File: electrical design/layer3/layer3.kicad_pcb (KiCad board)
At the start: 2 copper layers, 150 x 140 mm, 58 parts, among them J1 XT60PW-M, J10 SH1.0 Female, J11 SH1.0 Female, J12 MOTOR1, J13 MOTOR2, J14 MOTOR3, J15 MOTOR4, J16 CAMERA, J17 SH1.0 3P, J2 XT60PW-M, J3 XT30UPB-F, J4 XT30UPB-F, J5 XT30UPB-F, J6 XT30UPB-F, J7 XT30UPB-F, J8 COMPASS, J9 SH1.0 5P, SW1 SW_DPDT_x2, SW2 SW_Push, SW3 SW_DPDT_x2, SW4 SW_Push, U1 TEENSY 4.0, U2 STM32F103C8T6, U3 STM32F103C8T6, U4 74LVC2G04, U5 74LVC2G04, Y1 Crystal, Y2 Crystal

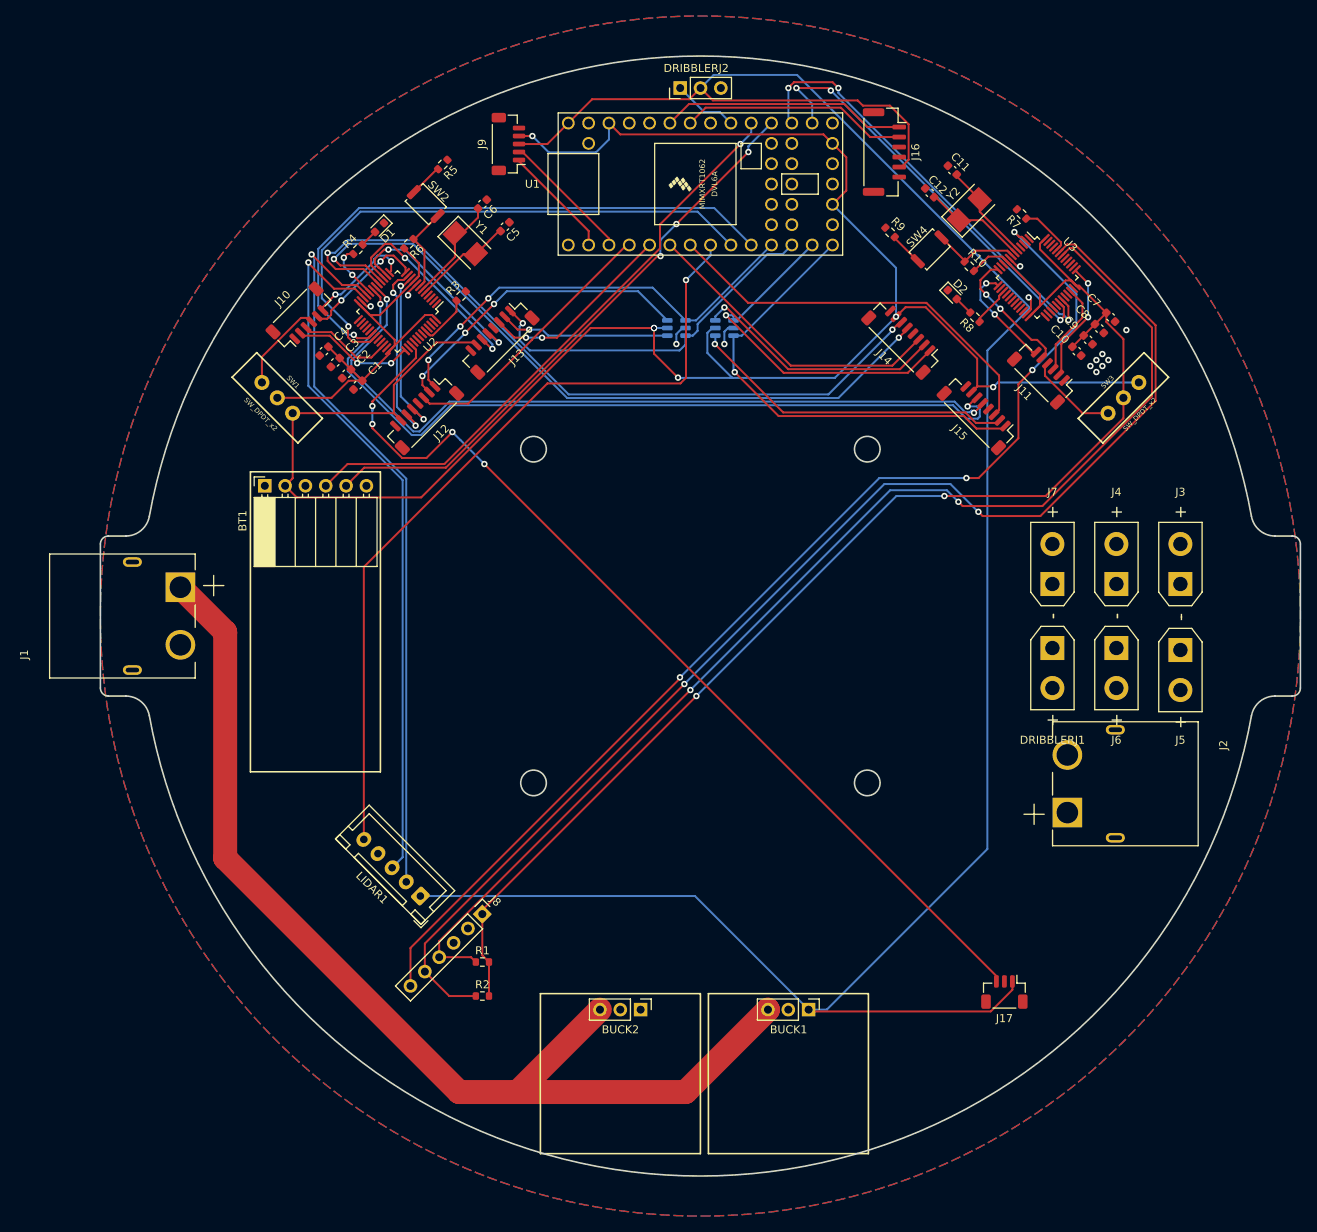
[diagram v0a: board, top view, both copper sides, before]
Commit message: submit all pcbs for production
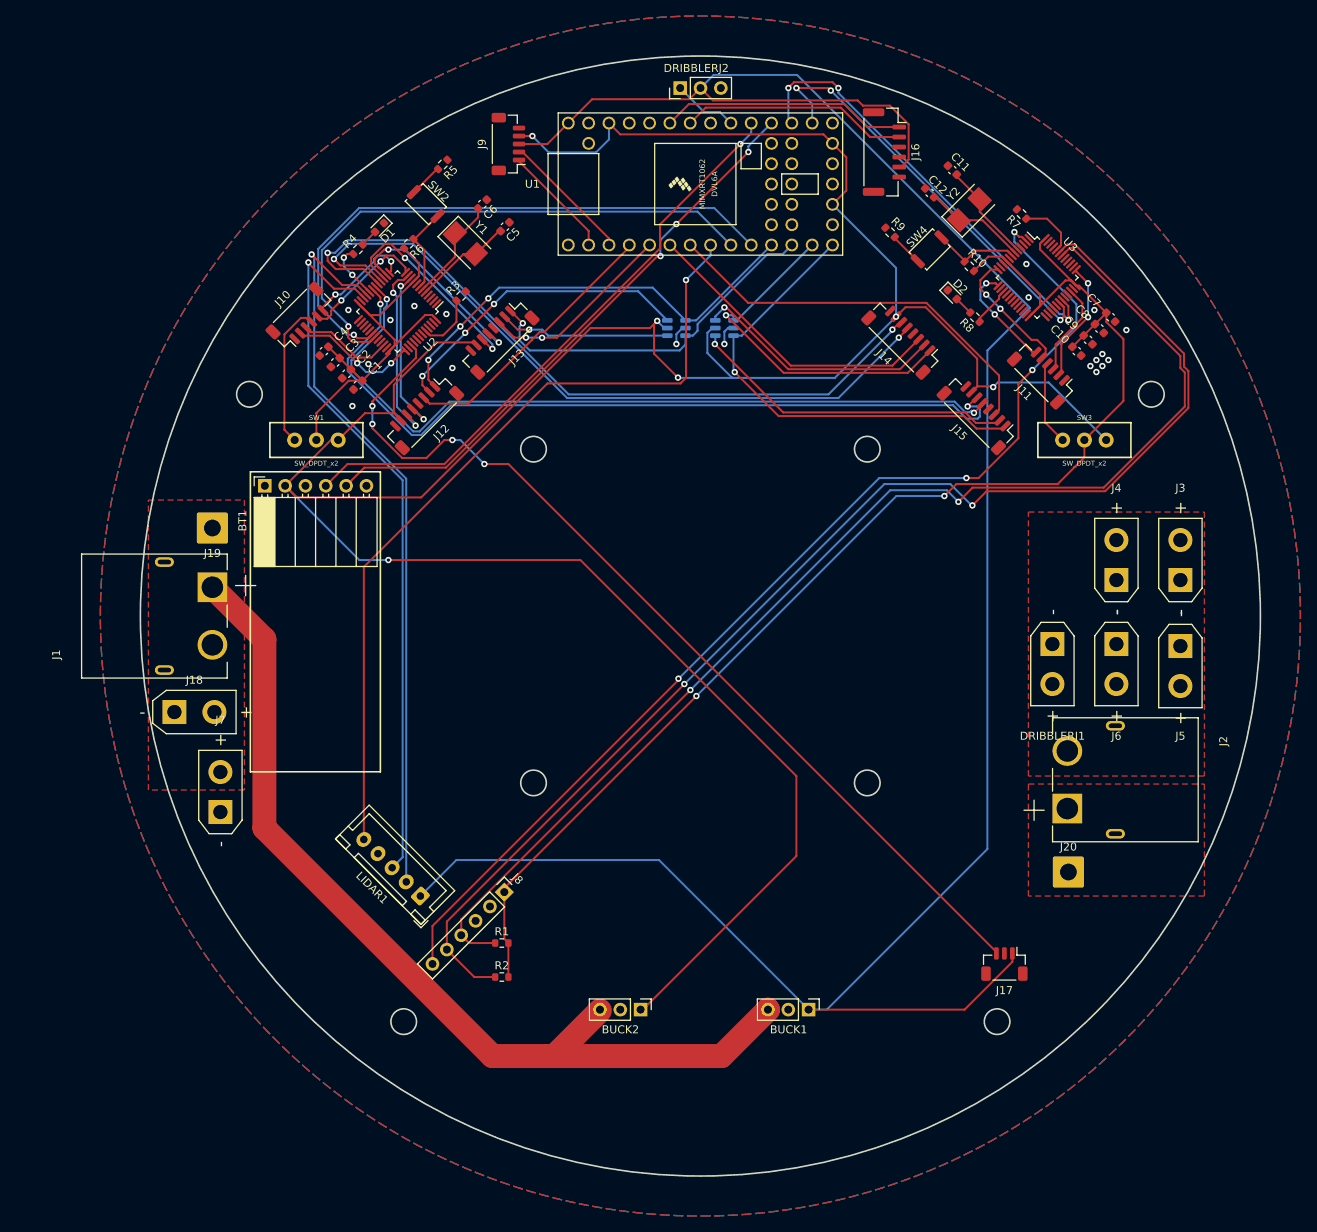
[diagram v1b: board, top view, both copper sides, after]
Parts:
- added J18: XT30UPB-F, Connector_AMASS:AMASS_XT30UPB-F_1x02_P5.0mm_Vertical, F.Cu at (44.2, 122.0)
- added J19: Conn_01x01_Female, Connector_Wire:SolderWire-1.5sqmm_1x01_D1.7mm_OD3.9mm, F.Cu at (49.0, 99.0)
- added J20: Conn_01x01_Female, Connector_Wire:SolderWire-1.5sqmm_1x01_D1.7mm_OD3.9mm, F.Cu at (156.0, 142.0)
- moved J7 107.8 mm to (50.0, 134.5)
- moved SW1 7.19 mm to (62.0, 88.0), turned to -90 degrees
- moved SW3 7.18 mm to (158.0, 88.0), turned to -90 degrees
- moved J1 4.00 mm to (43.0, 110.0)
- moved J8 3.89 mm to (85.5, 144.5)
- moved J17 3.50 mm to (148.0, 153.5)
- moved R1 3.39 mm to (85.2, 150.9)
- moved R2 3.39 mm to (85.2, 155.1)
- moved DRIBBLERJ1 0.50 mm to (154.0, 113.5)
- moved J2 0.50 mm to (161.9, 130.5)
- moved J3 0.50 mm to (170.0, 105.5)
- moved J4 0.50 mm to (162.0, 105.5)
- moved J5 0.50 mm to (170.0, 113.8)
- moved J6 0.50 mm to (162.0, 113.5)
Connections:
- J2 pad 1: +12V -> /BATT_+12V
- J2 pad 2: /BATT_+12V -> +12V
- J7 pad 2: +12V -> /BATT_+12V
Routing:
- net +3V3: track 251.6 -> 363.7 mm
- net /BATT_+12V: track 135.0 -> 118.5 mm
- net GND: track 13.1 -> 5.57 mm, vias 13 -> 19
- net /PROG3V31: track 11.6 -> 18.2 mm
- net +5V: track 296.0 -> 301.0 mm
- net /IMURST: track 141.2 -> 137.3 mm
- net /MCU3V32: track 172.3 -> 168.6 mm
- net /NEOPIXELOUT: track 123.0 -> 120.4 mm
- net /IMUSCL: track 150.1 -> 152.2 mm
- net /IMUSDA: track 160.1 -> 161.2 mm
- net /SWDCLOCK1: track 15.3 -> 16.3 mm
- net /PROG3V32: track 11.5 -> 10.6 mm
- net Net-(R3-Pad1): track 6.89 -> 7.64 mm
- net /MCU3V31: track 53.1 -> 52.3 mm
- net Net-(R7-Pad1): track 6.74 -> 7.45 mm
- added copper zone on F.Cu, net +12V
- added copper zone on F.Cu, net /BATT_+12V
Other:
- board size 150 x 140 mm -> 140 x 140 mm
